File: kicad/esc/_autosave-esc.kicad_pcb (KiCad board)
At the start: 2 copper layers, 83 parts, among them Q1 IRF540N, Q2 IRF540N, Q3 IRF540N, Q4 IRF540N, Q5 IRF540N, Q6 IRF540N, Q7 2N3904, U1 IR2110, U10 4N35, U11 4N35, U12 4N35, U13 4N35, U14 4N35, U15 4N35, U2 IR2110, U3 IR2110, U4 LM393, U5 LM393, U6 LM7805_TO220, U7 4N35, U8 4N35, U9 4N35

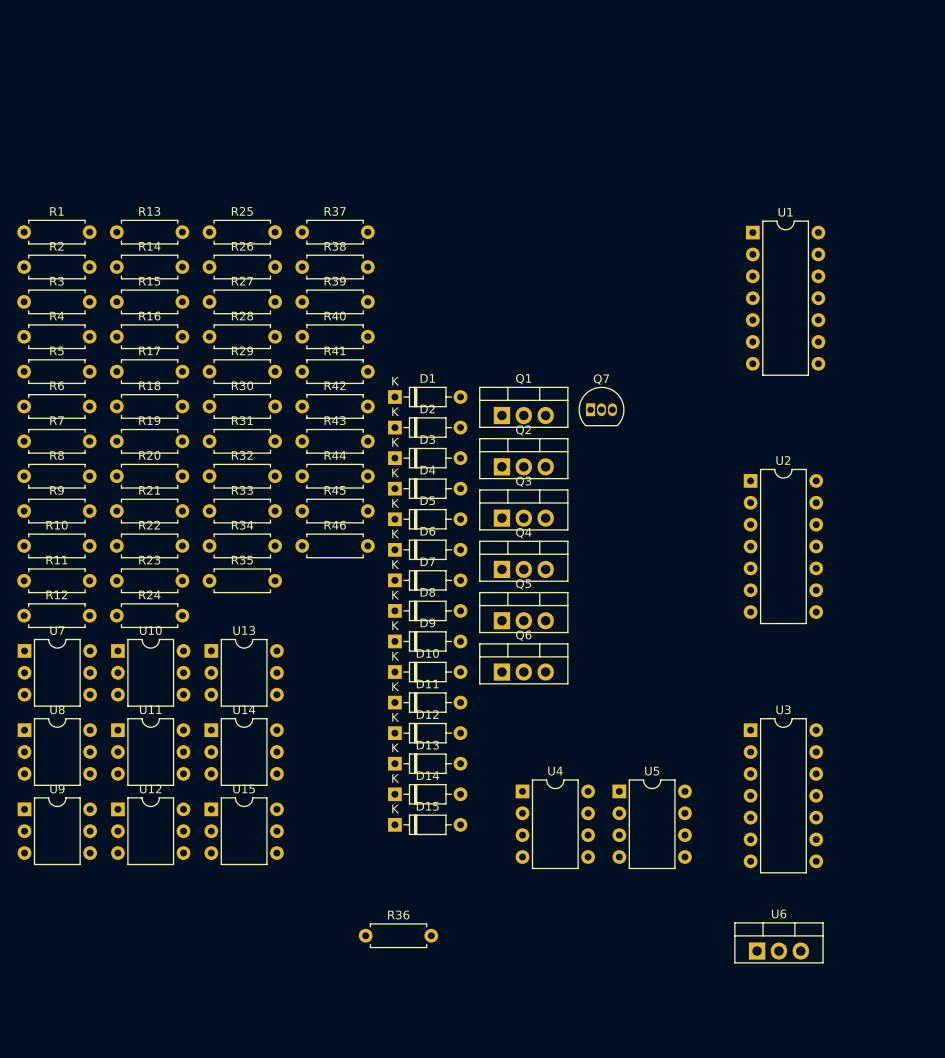
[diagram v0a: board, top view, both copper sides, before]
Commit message: RC1
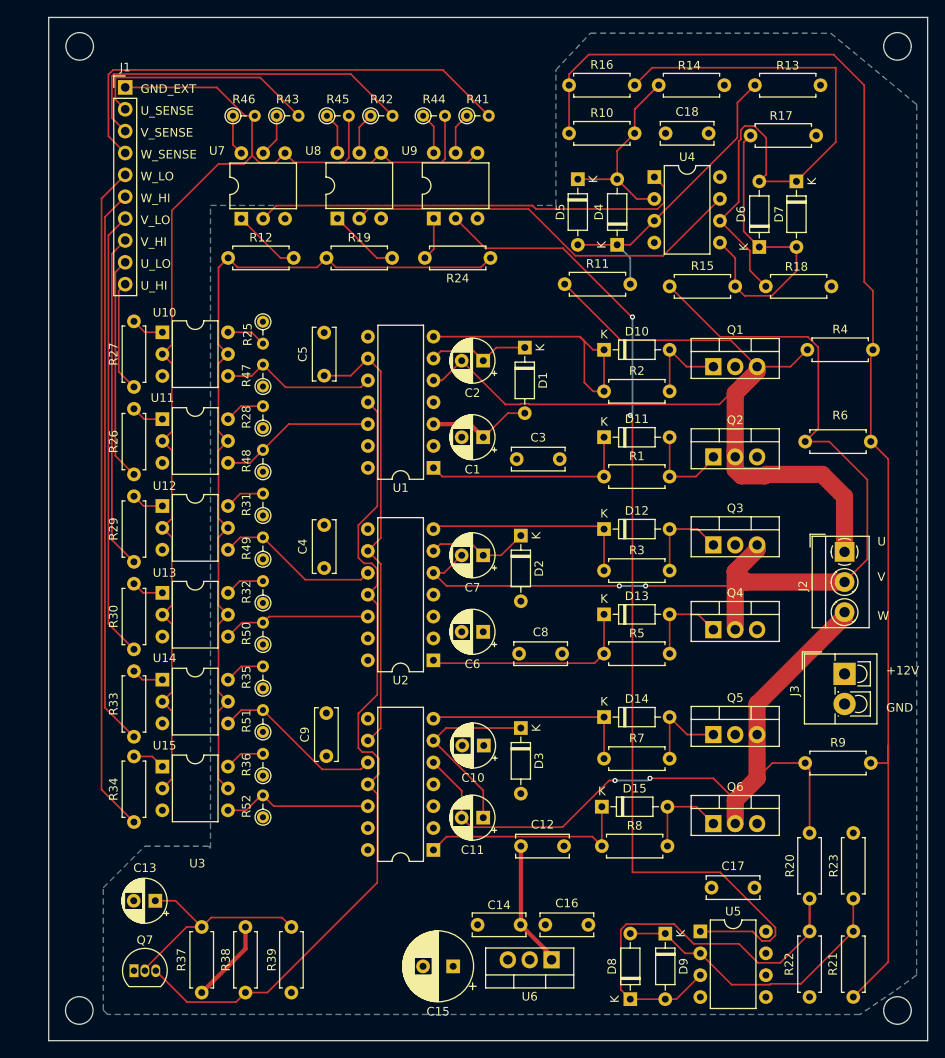
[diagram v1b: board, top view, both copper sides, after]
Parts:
- removed R40: 6.8k, Resistor_THT:R_Axial_DIN0207_L6.3mm_D2.5mm_P7.62mm_Horizontal
- added C1: 1u, Capacitor_THT:CP_Radial_D5.0mm_P2.50mm, F.Cu at (75.9, 73.4)
- added C10: 1u, Capacitor_THT:CP_Radial_D5.0mm_P2.50mm, F.Cu at (75.9, 109.2)
- added C11: 1u, Capacitor_THT:CP_Radial_D5.0mm_P2.50mm, F.Cu at (75.9, 117.6)
- added C12: 100n, Capacitor_THT:C_Disc_D6.0mm_W2.5mm_P5.00mm, F.Cu at (80.3, 120.9)
- added C13: 10u, Capacitor_THT:CP_Radial_D5.0mm_P2.50mm, F.Cu at (37.8, 127.3)
- added C14: 100n, Capacitor_THT:C_Disc_D6.0mm_W2.5mm_P5.00mm, F.Cu at (80.2, 130.0)
- added C15: 100u, Capacitor_THT:CP_Radial_D8.0mm_P3.50mm, F.Cu at (72.4, 134.9)
- added C16: 100n, Capacitor_THT:C_Disc_D6.0mm_W2.5mm_P5.00mm, F.Cu at (83.1, 130.0)
- added C17: 100n, Capacitor_THT:C_Disc_D6.0mm_W2.5mm_P5.00mm, F.Cu at (102.4, 125.7)
- added C18: 100n, Capacitor_THT:C_Disc_D6.0mm_W2.5mm_P5.00mm, F.Cu at (97.1, 38.1)
- added C2: 1u, Capacitor_THT:CP_Radial_D5.0mm_P2.50mm, F.Cu at (75.9, 64.5)
- added C3: 100n, Capacitor_THT:C_Disc_D6.0mm_W2.5mm_P5.00mm, F.Cu at (79.8, 75.9)
- added C4: 100n, Capacitor_THT:C_Disc_D6.0mm_W2.5mm_P5.00mm, F.Cu at (57.4, 88.6)
- added C5: 100n, Capacitor_THT:C_Disc_D6.0mm_W2.5mm_P5.00mm, F.Cu at (57.4, 66.3)
- added C6: 1u, Capacitor_THT:CP_Radial_D5.0mm_P2.50mm, F.Cu at (75.9, 96.0)
- added C7: 1u, Capacitor_THT:CP_Radial_D5.0mm_P2.50mm, F.Cu at (75.9, 87.1)
- added C8: 100n, Capacitor_THT:C_Disc_D6.0mm_W2.5mm_P5.00mm, F.Cu at (80.0, 98.6)
- added C9: 100n, Capacitor_THT:C_Disc_D6.0mm_W2.5mm_P5.00mm, F.Cu at (57.7, 110.5)
- added J1: ~, Connector_PinHeader_2.54mm:PinHeader_1x10_P2.54mm_Vertical, F.Cu at (34.3, 32.8)
- added J2: Motor, TerminalBlock_MetzConnect:TerminalBlock_MetzConnect_Type059_RT06303HBWC_1x03_P3.50mm_Horizontal, F.Cu at (117.9, 86.7)
- added J3: Screw_Terminal_01x02, TerminalBlock_4Ucon:TerminalBlock_4Ucon_1x02_P3.50mm_Vertical, F.Cu at (117.9, 100.9)
- added R47: 1k, Resistor_THT:R_Axial_DIN0204_L3.6mm_D1.6mm_P2.54mm_Vertical, F.Cu at (50.3, 67.5)
- added R48: 1k, Resistor_THT:R_Axial_DIN0204_L3.6mm_D1.6mm_P2.54mm_Vertical, F.Cu at (50.3, 77.4)
- added R49: 10k, Resistor_THT:R_Axial_DIN0204_L3.6mm_D1.6mm_P2.54mm_Vertical, F.Cu at (50.3, 87.6)
- added R50: 1k, Resistor_THT:R_Axial_DIN0204_L3.6mm_D1.6mm_P2.54mm_Vertical, F.Cu at (50.3, 97.5)
- added R51: 1k, Resistor_THT:R_Axial_DIN0204_L3.6mm_D1.6mm_P2.54mm_Vertical, F.Cu at (50.3, 107.6)
- added R52: 1k, Resistor_THT:R_Axial_DIN0204_L3.6mm_D1.6mm_P2.54mm_Vertical, F.Cu at (50.3, 117.6)
- added REF**: MountingHole_3.2mm_M3, MountingHole:MountingHole_3.2mm_M3, F.Cu at (29.0, 140.0)
- added REF**: MountingHole_3.2mm_M3, MountingHole:MountingHole_3.2mm_M3, F.Cu at (124.0, 140.0)
- added REF**: MountingHole_3.2mm_M3, MountingHole:MountingHole_3.2mm_M3, F.Cu at (29.0, 28.0)
- added REF**: MountingHole_3.2mm_M3, MountingHole:MountingHole_3.2mm_M3, F.Cu at (124.0, 28.0)
- R25, R28, R31, R32, R35, R36, R41, R42, R43, R44, R45, R46: footprint Resistor_THT:R_Axial_DIN0207_L6.3mm_D2.5mm_P7.62mm_Horizontal -> Resistor_THT:R_Axial_DIN0204_L3.6mm_D1.6mm_P2.54mm_Vertical
- R37: value 300k -> 330k
- moved R21 102.5 mm to (118.9, 138.4), turned to 90 degrees
- moved R22 96.0 mm to (113.8, 138.4), turned to 90 degrees
- moved R9 95.3 mm to (113.3, 111.3)
- moved R4 91.0 mm to (113.5, 63.2)
- moved R6 90.8 mm to (113.3, 73.9)
- moved R20 90.5 mm to (113.8, 119.4), turned to -90 degrees
- moved R23 90.4 mm to (118.9, 119.4), turned to -90 degrees
- moved R37 89.1 mm to (43.2, 137.9), turned to 90 degrees
- moved R17 85.7 mm to (114.6, 38.4), turned to 180 degrees
- moved R18 84.2 mm to (116.3, 55.9), turned to 180 degrees
- moved Q7 84.0 mm to (35.3, 135.4)
- moved R13 83.5 mm to (115.1, 32.5), turned to 180 degrees
- moved U9 83.5 mm to (70.1, 48.0), turned to 90 degrees
- moved R8 79.7 mm to (89.7, 120.9)
- moved R10 79.4 mm to (85.9, 38.1)
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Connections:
- Q7 pad 3: +12V -> Net-(Q7-C)
- R37 pad 1: +12V -> +5V
- R38 pad 1: +12V -> +5V
- R38 pad 2: +12V -> Net-(Q7-C)
- U1 pad 11: +12V -> Net-(Q7-C)
- U2 pad 11: +12V -> Net-(Q7-C)
- U3 pad 11: +12V -> Net-(Q7-C)
- U5 pad 5: (no net) -> GND
- U5 pad 6: (no net) -> GND
- U5 pad 7: (no net) -> GND
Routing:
- net +5V: track 0.00 -> 162.0 mm
- net Net-(R10-Pad1): track 0.00 -> 156.6 mm
- net GND_EXT: track 0.00 -> 145.8 mm
- net Net-(U5-Pad1): track 0.00 -> 119.6 mm, vias 0 -> 2
- net V: track 0.00 -> 118.0 mm, vias 0 -> 2
- net U: track 0.00 -> 109.8 mm
- net Net-(Q7-C): track 0.00 -> 96.1 mm
- net W: track 0.00 -> 88.4 mm, vias 0 -> 2
- net W_LO: track 0.00 -> 77.9 mm
- net Net-(D6-A): track 0.00 -> 74.1 mm
- net W_HI: track 0.00 -> 65.1 mm
- net W_SENSE: track 0.00 -> 56.5 mm
- net V_LO: track 0.00 -> 52.1 mm
- net Net-(D8-K): track 0.00 -> 51.2 mm
- net Net-(U4-Pad1): track 0.00 -> 51.1 mm
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- added copper zone on In2.Cu, net +12V
- added copper zone on In2.Cu, net +5V
- added copper zone on B.Cu, net GND
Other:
- board outline added: 102.1 x 118.9 mm
- copper layers 2 -> 4
- board text added: "+12V"
- board text added: "GND"
- board text added: "GND_EXT"
- board text added: "U"
- board text added: "U_HI"
- board text added: "U_LO"
- board text added: "U_SENSE"
- board text added: "V"
- board text added: "V_HI"
- board text added: "V_LO"
- board text added: "V_SENSE"
- board text added: "W"
- board text added: "W_HI"
- board text added: "W_LO"
- board text added: "W_SENSE"
